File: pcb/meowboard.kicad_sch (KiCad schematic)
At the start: 101 parts, among them SW1 SW_Push_45deg, SW10 SW_Push_45deg, SW11 SW_Push_45deg, SW12 SW_Push_45deg, SW14 SW_Push_45deg, SW15 SW_Push_45deg, SW16 SW_Push_45deg, SW17 SW_Push_45deg, SW18 SW_Push_45deg, SW19 SW_Push_45deg, SW2 SW_Push_45deg, SW20 SW_Push_45deg, SW21 SW_Push_45deg, SW22 SW_Push_45deg, SW23 SW_Push_45deg, SW24 SW_Push_45deg, SW25 SW_Push_45deg, SW26 SW_Push_45deg, SW27 SW_Push_45deg, SW28 SW_Push_45deg, SW29 SW_Push_45deg, SW3 SW_Push_45deg, SW30 SW_Push_45deg, SW31 SW_Push_45deg, SW32 SW_Push_45deg, SW33 SW_Push_45deg, SW34 SW_Push_45deg, SW35 SW_Push_45deg, SW36 SW_Push_45deg, SW37 SW_Push_45deg, SW38 SW_Push_45deg, SW39 SW_Push_45deg, SW4 SW_Push_45deg, SW40 SW_Push_45deg, SW41 SW_Push_45deg, SW42 SW_Push_45deg, SW43 SW_Push_45deg, SW45 SW_Push_45deg, SW46 SW_Push_45deg, SW47 SW_Push_45deg, SW48 SW_Push_45deg, SW49 SW_Push_45deg, SW5 SW_Push_45deg, SW50 SW_Push_45deg, SW51 SW_Push_45deg, SW52 SW_Push_45deg, SW6 SW_Push_45deg, SW7 SW_Push_45deg, SW8 SW_Push_45deg, SW9 SW_Push_45deg, U1 Pico

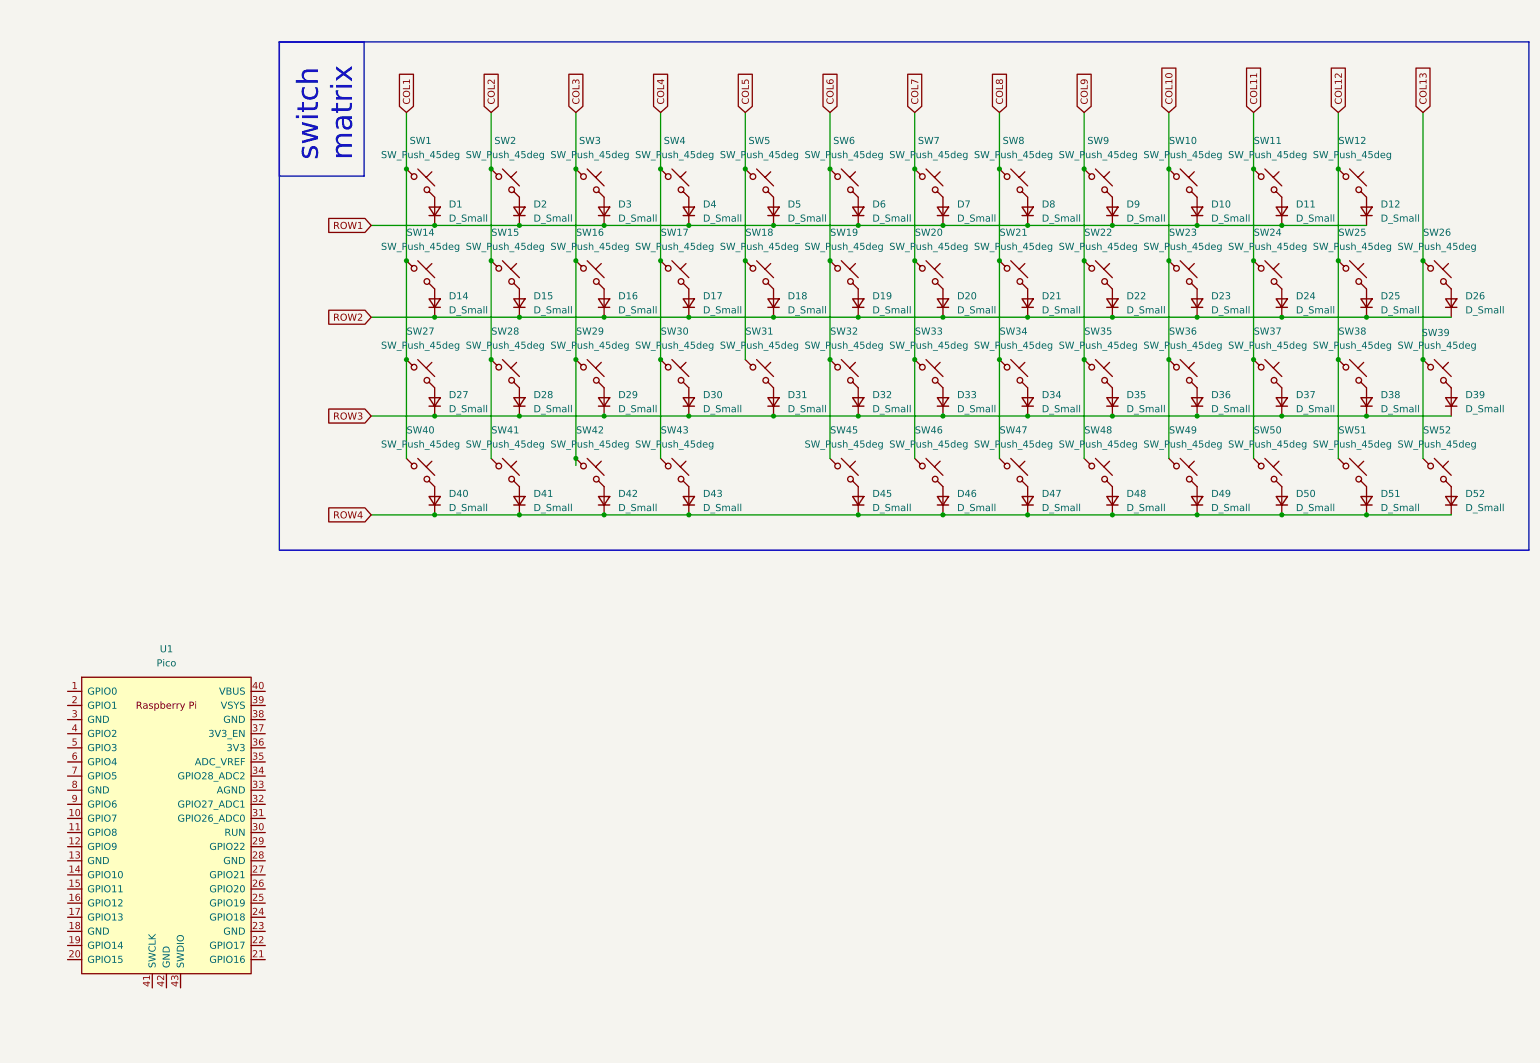
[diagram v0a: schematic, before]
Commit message: updates
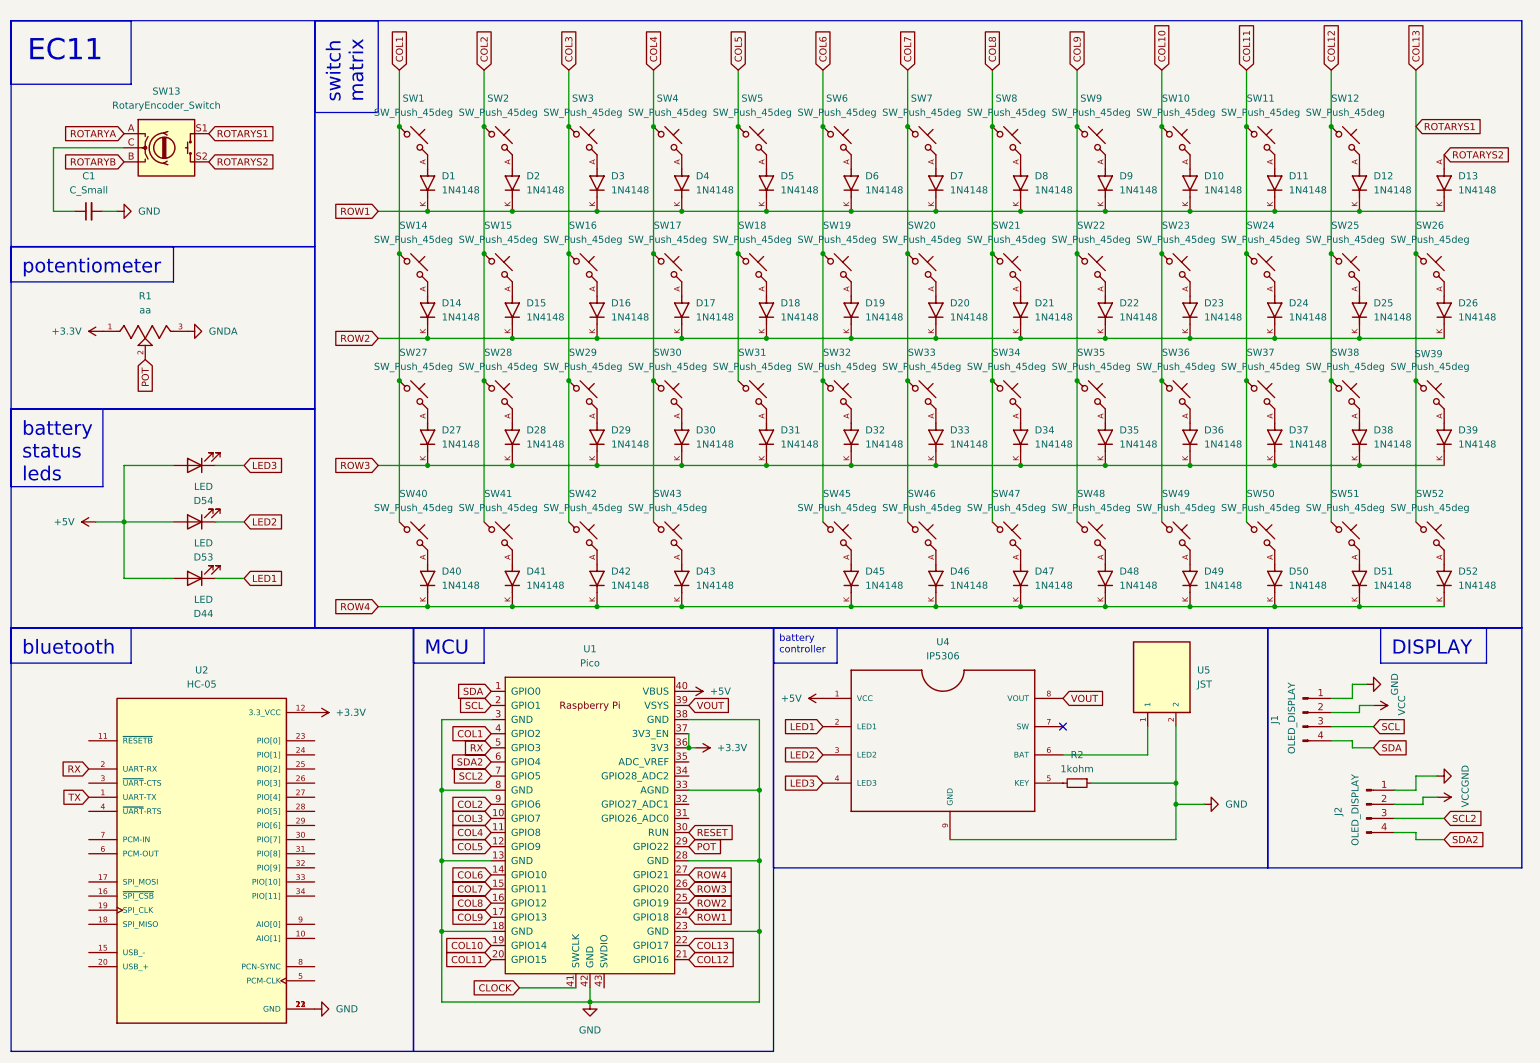
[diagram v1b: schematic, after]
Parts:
- removed D1, D10, D11, D12, D14, D15, D16, D17, D18, D19, D2, D20, D21, D22, D23, D24, D25, D26, D27, D28, D29, D3, D30, D31, D32, D33, D34, D35, D36, D37, D38, D39, D4, D40, D41, D42, D43, D45, D46, D47, D48, D49, D5, D50, D51, D52, D6, D7, D8, D9: D_Small, symbol Device:D_Small
- added C1: C_Small, Capacitor_THT:CP_Radial_D4.0mm_P1.50mm, symbol Device:C_Small
- added D1, D10, D11, D12, D13, D14, D15, D16, D17, D18, D19, D2, D20, D21, D22, D23, D24, D25, D26, D27, D28, D29, D3, D30, D31, D32, D33, D34, D35, D36, D37, D38, D39, D4, D40, D41, D42, D43, D45, D46, D47, D48, D49, D5, D50, D51, D52, D6, D7, D8, D9: 1N4148, 1N4148:DIOAD753W49L380D172B, symbol 1N4148:1N4148
- added D44, D53, D54: LED, LED_THT:LED_D1.8mm_W1.8mm_H2.4mm_Horizontal_O1.27mm_Z1.6mm, symbol Device:LED
- added J1, J2: OLED_DISPLAY, oled:SSD1306-0.91-OLED-4pin-128x32, symbol Connector:Conn_01x04_Pin
- added R1: aa, 3310Y-001-103L:TRIM_3310Y-001-103L, symbol 3310Y-001-103L:3310Y-001-103L
- added R2: 1kohm, Resistor_THT:R_Axial_DIN0204_L3.6mm_D1.6mm_P1.90mm_Vertical, symbol Device:R_Small
- added SW13: RotaryEncoder_Switch, Rotaries:RotaryEncoder_Alps_EC11E-Switch_Vertical_H20mm, symbol Device:RotaryEncoder_Switch
- added U2: HC-05, HC-05:XCVR_HC-05, symbol HC-05:HC-05
- added U4: IP5306, IP5306:SOIC9P127_490X600X170L84X42T330X241N, symbol IP5306:IP5306
- added U5: JST, B2B-PH-SM4-TB:SM4-CON, symbol B2B-PH-SM4-TB_LF__SN_:B2B-PH-SM4-TB_LF__SN_
- SW1, SW10, SW11, SW14, SW15, SW16, SW17, SW18, SW19, SW2, SW20, SW21, SW22, SW23, SW24, SW25, SW26, SW27, SW28, SW29, SW3, SW30, SW31, SW32, SW33, SW34, SW35, SW36, SW37, SW38, SW39, SW4, SW40, SW41, SW42, SW45, SW46, SW47, SW48, SW49, SW5, SW50, SW51, SW52, SW6, SW7, SW8, SW9: footprint (none) -> MX_Hotswap:MX-Hotswap-1U
- SW12, SW43: footprint (none) -> MX_Hotswap:MX-Hotswap-2U
- U1: footprint RPi_Pico:RPi_Pico_SMD_TH -> Pico:RPi_Pico_SMD_TH
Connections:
- net COL1: now also U1.4 (GPIO2)
- net COL10: now also U1.19 (GPIO14)
- net COL11: now also U1.20 (GPIO15)
- net COL12: now also U1.21 (GPIO16)
- net COL13: now also U1.22 (GPIO17), SW13.S1
- net COL2: now also U1.9 (GPIO6)
- net COL3: now also U1.10 (GPIO7)
- net COL4: now also U1.11 (GPIO8)
- net COL5: now also U1.12 (GPIO9)
- net COL6: now also U1.14 (GPIO10)
- net COL7: now also U1.15 (GPIO11)
- net COL8: now also U1.16 (GPIO12)
- net COL9: now also U1.17 (GPIO13)
- net ROW1: now also U1.24 (GPIO18), D1.K, D10.K, D11.K, D12.K, D13.K, D2.K, D3.K, D4.K, D5.K, D6.K, D7.K, D8.K, D9.K
- net ROW2: now also U1.25 (GPIO19), D14.K, D15.K, D16.K, D17.K, D18.K, D19.K, D20.K, D21.K, D22.K, D23.K, D24.K, D25.K, D26.K
- net ROW3: now also U1.26 (GPIO20), D27.K, D28.K, D29.K, D30.K, D31.K, D32.K, D33.K, D34.K, D35.K, D36.K, D37.K, D38.K, D39.K
- net ROW4: now also U1.27 (GPIO21), D40.K, D41.K, D42.K, D43.K, D45.K, D46.K, D47.K, D48.K, D49.K, D50.K, D51.K, D52.K
- net at SW52.2: now also D52.A
- net SDA: now reaches U1.1 (GPIO0)
- net SDA: now also J1.4 (Pin_4)
- net GND: now reaches U1.13 (GND)
- net GND: now also U1.18 (GND), U1.23 (GND), U1.28 (GND), U1.3 (GND), U1.33 (AGND), U1.38 (GND), U1.42 (GND), U1.8 (GND), C1.2, J1.1 (Pin_1), J2.1 (Pin_1), R2.1, U2.13 (GND), U2.21 (GND), U2.22 (GND), U4.9 (GND), U5.2
- net SCL: now reaches U1.2 (GPIO1)
- net SCL: now also J1.3 (Pin_3)
- net POT: now reaches U1.29 (GPIO22)
- net POT: now also R1.2
- net RESET: now reaches U1.30 (RUN)
- net +3.3V: now reaches U1.36 (3V3)
- net +3.3V: now also U1.37 (3V3_EN), R1.1, U2.12 (3.3_VCC)
- net VOUT: now reaches U1.39 (VSYS)
- net VOUT: now also U4.8 (VOUT)
- net +5V: now reaches U1.40 (VBUS)
- net +5V: now also D44.2 (A), D53.2 (A), D54.2 (A), U4.1 (VCC)
- net CLOCK: now reaches U1.41 (SWCLK)
- net RX: now reaches U1.5 (GPIO3)
- net RX: now also U2.2 (UART-RX)
- net SDA2: now reaches U1.6 (GPIO4)
- net SDA2: now also J2.4 (Pin_4)
- net SCL2: now reaches U1.7 (GPIO5)
- net SCL2: now also J2.3 (Pin_3)
- net at SW7.2: now also D7.A
- net at SW28.2: now also D28.A
- net at SW8.2: now also D8.A
- net at SW18.2: now also D18.A
- net at SW21.2: now also D21.A
- net at SW40.2: now also D40.A
- net at SW26.2: now also D26.A
- net at SW2.2: now also D2.A
- net at SW31.2: now also D31.A
- net at SW42.2: now also D42.A
- net at SW15.2: now also D15.A
- net at SW5.2: now also D5.A
- net at SW36.2: now also D36.A
- net at SW41.2: now also D41.A
- net at SW6.2: now also D6.A
- net at SW20.2: now also D20.A
- net at SW39.2: now also D39.A
- net at SW35.2: now also D35.A
- net at SW49.2: now also D49.A
- net at SW48.2: now also D48.A
- net at SW25.2: now also D25.A
- net at SW37.2: now also D37.A
- net at SW9.2: now also D9.A
- net at SW1.2: now also D1.A
- net at SW11.2: now also D11.A
- net at SW22.2: now also D22.A
- net at SW46.2: now also D46.A
- net at SW33.2: now also D33.A
- net at SW47.2: now also D47.A
- net at SW16.2: now also D16.A
- net at SW32.2: now also D32.A
- net at SW19.2: now also D19.A
- net at SW38.2: now also D38.A
- net at SW4.2: now also D4.A
- net at SW34.2: now also D34.A
- net at SW23.2: now also D23.A
- net at SW12.2: now also D12.A
- net at SW29.2: now also D29.A
- net at SW14.2: now also D14.A
- net at SW27.2: now also D27.A
- net at SW50.2: now also D50.A
- net at SW51.2: now also D51.A
- net at SW30.2: now also D30.A
- net at SW17.2: now also D17.A
- net at SW45.2: now also D45.A
- net at SW24.2: now also D24.A
- net at SW3.2: now also D3.A
- net at SW43.2: now also D43.A
- net at SW10.2: now also D10.A
- new net: R2.2, U4.5 (KEY)
- new net: U4.6 (BAT), U5.1
- new net: C1.1, SW13.C
- new net GNDA: R1.3
- new net LED1: D44.1 (K), U4.2 (LED1)
- new net LED2: D53.1 (K), U4.3 (LED2)
- new net LED3: D54.1 (K), U4.4 (LED3)
- new net ROTARYA: SW13.A
- new net ROTARYB: SW13.B
- new net ROTARYS2: D13.A, SW13.S2
- new net TX: U2.1 (UART-TX)
- new net VCC: J1.2 (Pin_2), J2.2 (Pin_2)
- no-connect marks 0 -> 1
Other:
- moved on the sheet: SW1, SW10, SW11, SW12, SW14, SW15, SW16, SW17, SW18, SW19, SW2, SW20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
